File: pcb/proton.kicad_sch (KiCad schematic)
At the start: 5 parts, among them J1 Conn_01x28_Socket, J12 Conn_01x28_Socket, J13 Conn_01x04_Socket, J14 Conn_01x03_Socket, J6 691137710003

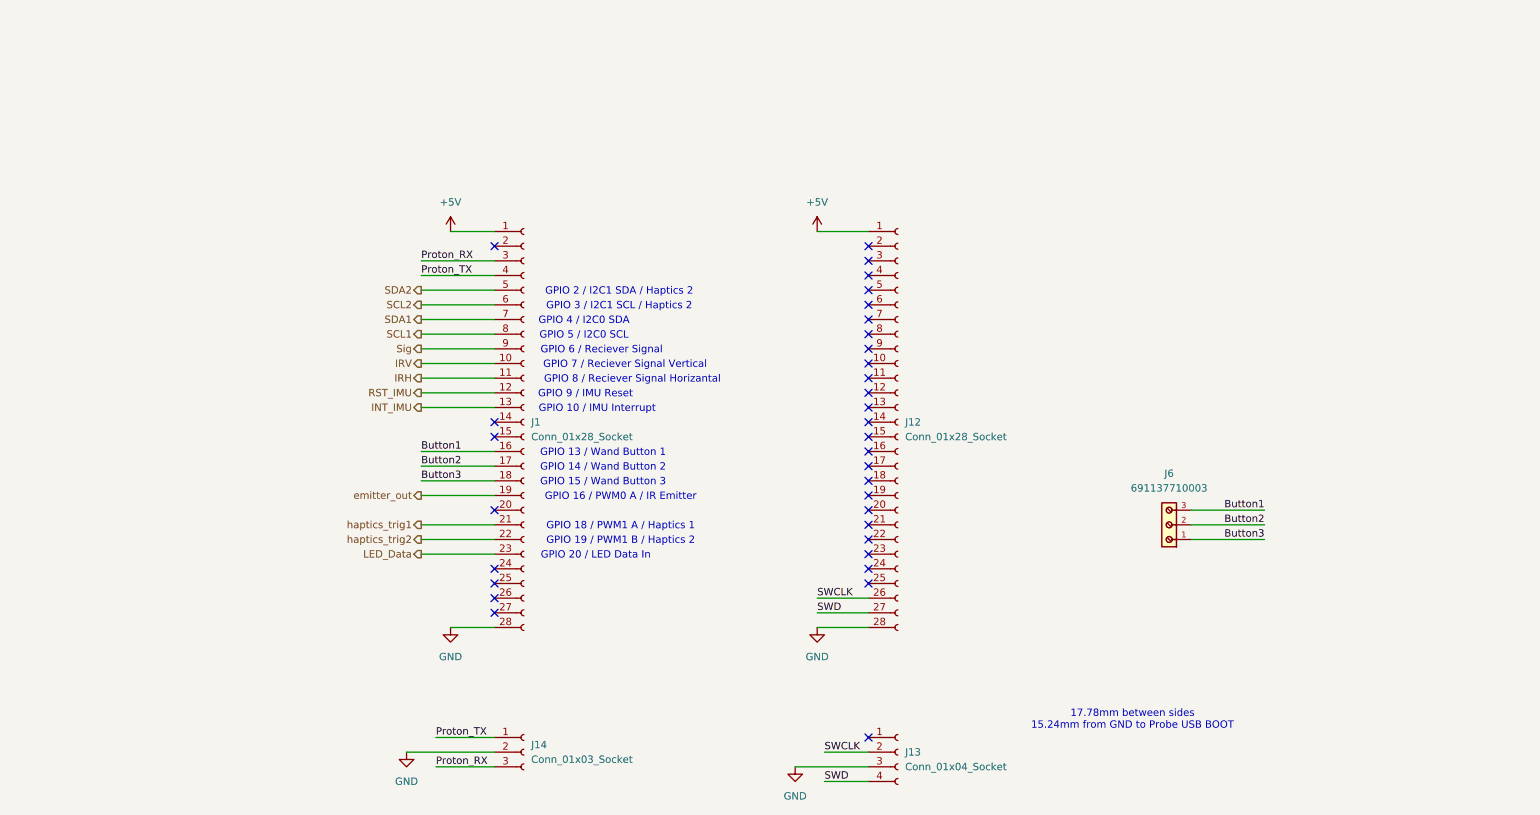
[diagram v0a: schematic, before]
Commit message: board
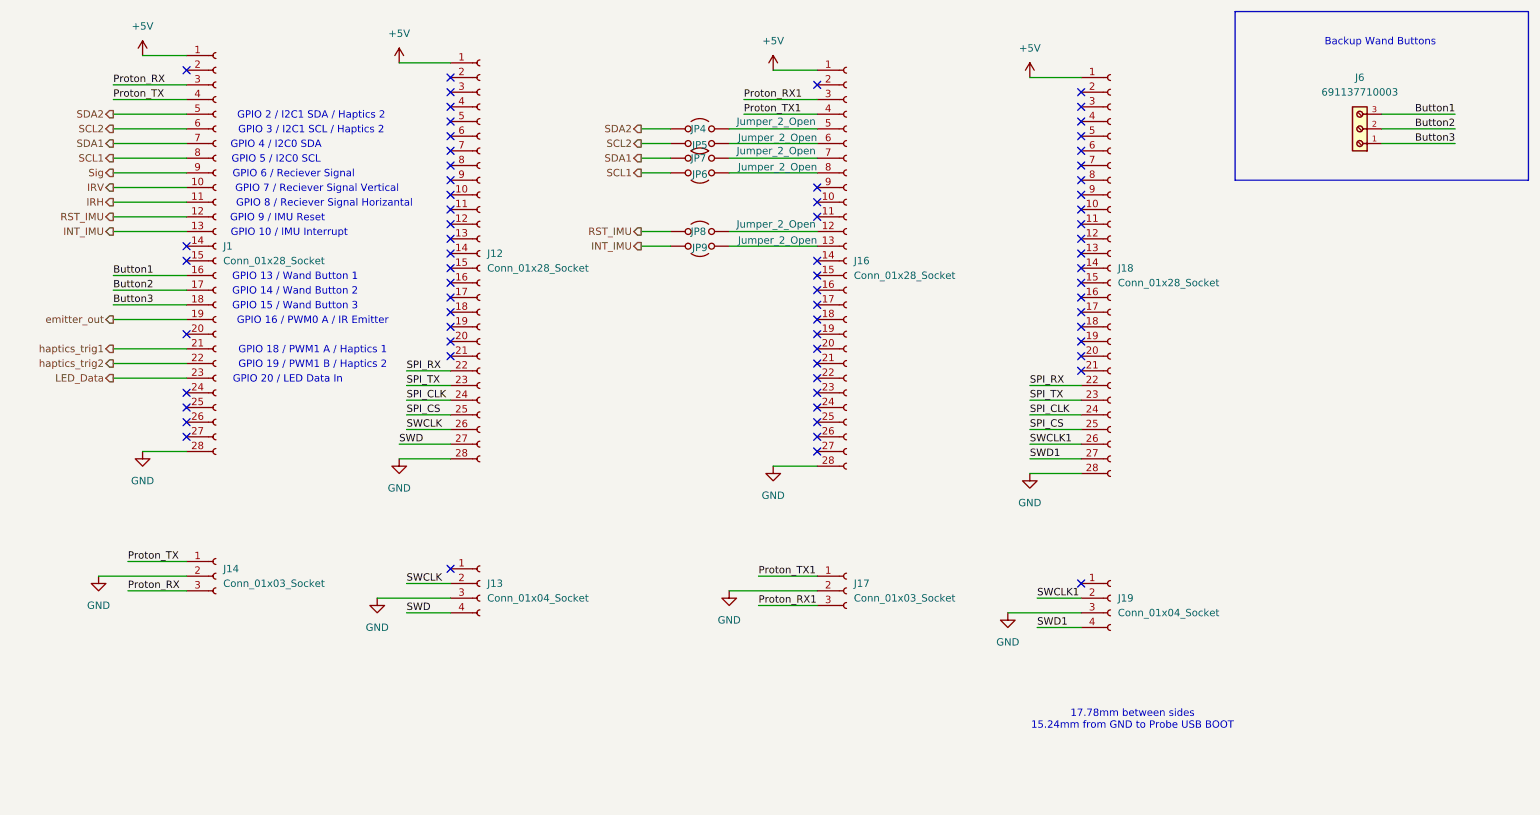
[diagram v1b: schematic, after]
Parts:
- added J16, J18: Conn_01x28_Socket, Connector_PinSocket_2.54mm:PinSocket_1x28_P2.54mm_Vertical, symbol Connector:Conn_01x28_Socket
- added J17: Conn_01x03_Socket, Connector_PinSocket_2.54mm:PinSocket_1x03_P2.54mm_Vertical, symbol Connector:Conn_01x03_Socket
- added J19: Conn_01x04_Socket, Connector_PinHeader_2.54mm:PinHeader_1x04_P2.54mm_Vertical, symbol Connector:Conn_01x04_Socket
- added JP4, JP5, JP6, JP7, JP8, JP9: Jumper_2_Open, TestPoint:TestPoint_2Pads_Pitch2.54mm_Drill0.8mm, symbol Jumper:Jumper_2_Open
- J14: footprint Connector_PinSocket_2.54mm:PinSocket_1x01_P2.54mm_Vertical -> Connector_PinSocket_2.54mm:PinSocket_1x03_P2.54mm_Vertical
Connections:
- net +5V: now also J16.1 (Pin_1), J18.1 (Pin_1)
- net GND: now also J16.28 (Pin_28), J17.2 (Pin_2), J18.28 (Pin_28), J19.3 (Pin_3)
- net INT_IMU: now also JP9.2 (B)
- net RST_IMU: now also JP8.1 (A)
- net SCL1: now also JP6.2 (B)
- net SCL2: now also JP5.2 (B)
- net SDA1: now also JP7.1 (A)
- net SDA2: now also JP4.1 (A)
- net SPI_RX: now reaches J12.22 (Pin_22)
- net SPI_RX: now also J18.22 (Pin_22)
- net SPI_TX: now reaches J12.23 (Pin_23)
- net SPI_TX: now also J18.23 (Pin_23)
- net SPI_CLK: now reaches J12.24 (Pin_24)
- net SPI_CLK: now also J18.24 (Pin_24)
- net SPI_CS: now reaches J12.25 (Pin_25)
- net SPI_CS: now also J18.25 (Pin_25)
- new net: J16.6 (Pin_6), JP5.1 (A)
- new net: J16.8 (Pin_8), JP6.1 (A)
- new net: J16.7 (Pin_7), JP7.2 (B)
- new net: J16.12 (Pin_12), JP8.2 (B)
- new net: J16.13 (Pin_13), JP9.1 (A)
- new net: J16.5 (Pin_5), JP4.2 (B)
- new net Proton_RX1: J16.3 (Pin_3), J17.3 (Pin_3)
- new net Proton_TX1: J16.4 (Pin_4), J17.1 (Pin_1)
- new net SWCLK1: J18.26 (Pin_26), J19.2 (Pin_2)
- new net SWD1: J18.27 (Pin_27), J19.4 (Pin_4)
- no-connect marks 33 -> 68
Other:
- note added: "Backup Wand Buttons"
- moved on the sheet: J1, J12, J13, J14, J6
